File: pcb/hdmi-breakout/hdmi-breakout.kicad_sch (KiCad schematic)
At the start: 4 parts, among them J1 Conn_01x09, J2 HDMI_A_1.4, J3 HDMI_A_1.4, J4 Conn_01x09

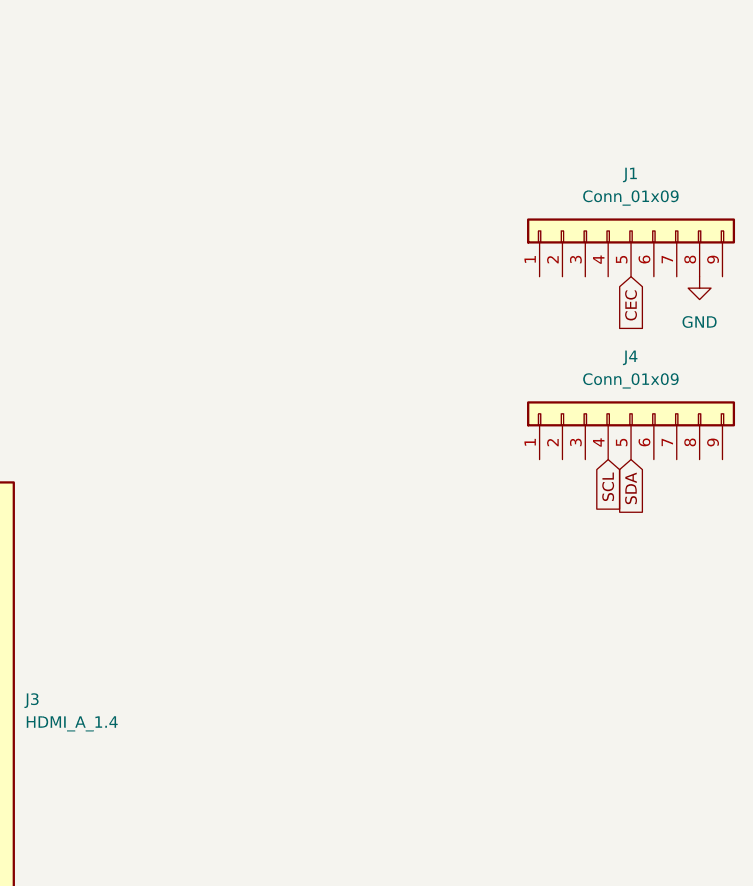
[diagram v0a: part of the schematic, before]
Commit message: correct hardware bugs
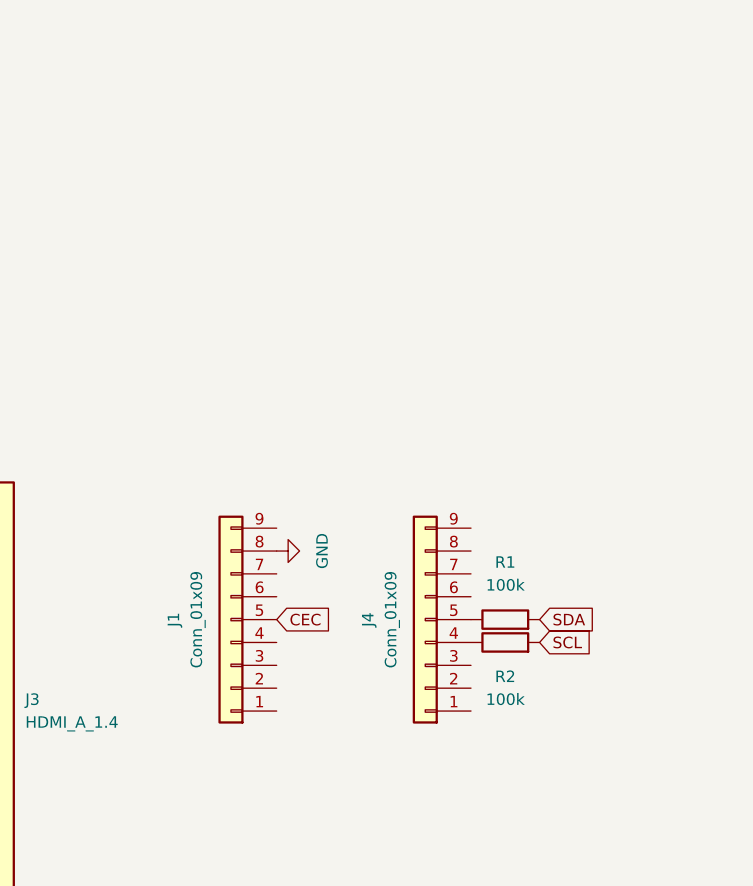
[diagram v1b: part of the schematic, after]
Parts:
- added R1, R2: 100k, Resistor_SMD:R_0603_1608Metric_Pad0.98x0.95mm_HandSolder, symbol Device:R
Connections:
- net SCL: now also R2.2; no longer J4.4 (Pin_4)
- net SDA: now also R1.2; no longer J4.5 (Pin_5)
- new net: J4.5 (Pin_5), R1.1
- new net: J4.4 (Pin_4), R2.1
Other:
- moved on the sheet: J1, J4

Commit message: update BOM
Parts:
- J1, J4: AVL1 (none) -> HCTL; AVL1 P/N (none) -> PM254-1-09-Z-8.5; LCSC (none) -> C2897372
- R1, R2: AVL1 (none) -> Uniroyal; AVL1 P/N (none) -> 0603WAF1003T5E; LCSC (none) -> C25803
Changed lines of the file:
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@@
+			)
+		)
+		(property "AVL1" "Uniroyal"
+			(at 224.79 69.85 90)
+			(hide yes)
+			(show_name no)
+			(do_not_autoplace no)
+			(effects
+				(font
+					(size 1.27 1.27)
+				)
+			)
+		)
+		(property "AVL1 P/N" "0603WAF1003T5E"
+			(at 224.79 69.85 90)
+			(hide yes)
+			(show_name no)
+			(do_not_autoplace no)
+			(effects
+				(font
+					(size 1.27 1.27)
+				)
+			)
+		)
+		(property "LCSC" "C25803"
+			(at 224.79 69.85 90)
+			(hide yes)
+			(show_name no)
+			(do_not_autoplace no)
+			(effects
+				(font
+					(size 1.27 1.27)
+				)
 			)
 		)
@@
 			)
 		)
+		(property "AVL1" "Uniroyal"
+			(at 224.79 72.39 90)
+			(hide yes)
+			(show_name no)
+			(do_not_autoplace no)
+			(effects
+				(font
+					(size 1.27 1.27)
+				)
+			)
+		)
+		(property "AVL1 P/N" "0603WAF1003T5E"
+			(at 224.79 72.39 90)
+			(hide yes)
+			(show_name no)
+			(do_not_autoplace no)
+			(effects
+				(font
+					(size 1.27 1.27)
+				)
+			)
+		)
+		(property "LCSC" "C25803"
+			(at 224.79 72.39 90)
+			(hide yes)
+			(show_name no)
+			(do_not_autoplace no)
+			(effects
+				(font
+					(size 1.27 1.27)
+				)
+			)
+		)
 		(pin "1"
 		)
@@
 			)
 		)
+		(property "LCSC" "C2897372"
+			(at 194.31 69.85 90)
+			(hide yes)
+			(show_name no)
+			(do_not_autoplace no)
+			(effects
+				(font
+					(size 1.27 1.27)
+				)
+			)
+		)
+		(property "AVL1" "HCTL"
+			(at 194.31 69.85 90)
+			(hide yes)
+			(show_name no)
+			(do_not_autoplace no)
+			(effects
+				(font
+					(size 1.27 1.27)
+				)
+			)
+		)
+		(property "AVL1 P/N" "PM254-1-09-Z-8.5"
+			(at 194.31 69.85 90)
+			(hide yes)
+			(show_name no)
+			(do_not_autoplace no)
+			(effects
+				(font
+					(size 1.27 1.27)
+				)
+			)
+		)
 		(pin "3"
 		)
@@
 			(hide yes)
 			(show_name no)
+			(do_not_autoplace no)
+			(effects
+				(font
+					(size 1.27 1.27)
+				)
+			)
+		)
+		(property "LCSC" "C2897372"
+			(at 215.9 69.85 90)
+			(hide yes)
+			(show_name no)
+			(do_not_autoplace no)
+			(effects
+				(font
+					(size 1.27 1.27)
+				)
+			)
+		)
+		(property "AVL1" "HCTL"
+			(at 215.9 69.85 90)
+			(hide yes)
+			(show_name no)
+			(do_not_autoplace no)
+			(effects
+				(font
+					(size 1.27 1.27)
+				)
+			)
+		)
+		(property "AVL1 P/N" "PM254-1-09-Z-8.5"
+			(at 215.9 69.85 90)
+			(hide yes)
+			(show_name no)
